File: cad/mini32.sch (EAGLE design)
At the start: 55 parts, among them CN1 MICROSDPLAIN, J1 HEADER-5X1, Q1 MOSFETSOT-23, SW2 SWITCHKMR211, SW3 SWITCHKMR211, U1 STM32F411/48, U2 LSM303D, U3 ADP5062, U4 MCP1824, U5 MAX17048, X1 12MHz, X2 32k768

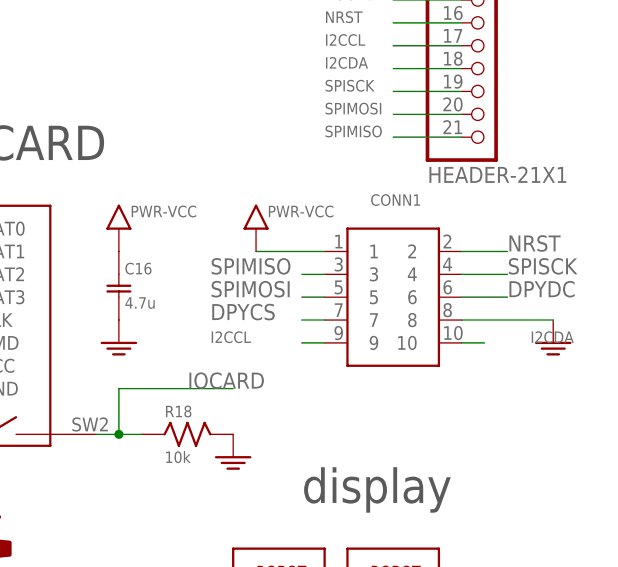
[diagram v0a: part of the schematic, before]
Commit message: 8pin dpy
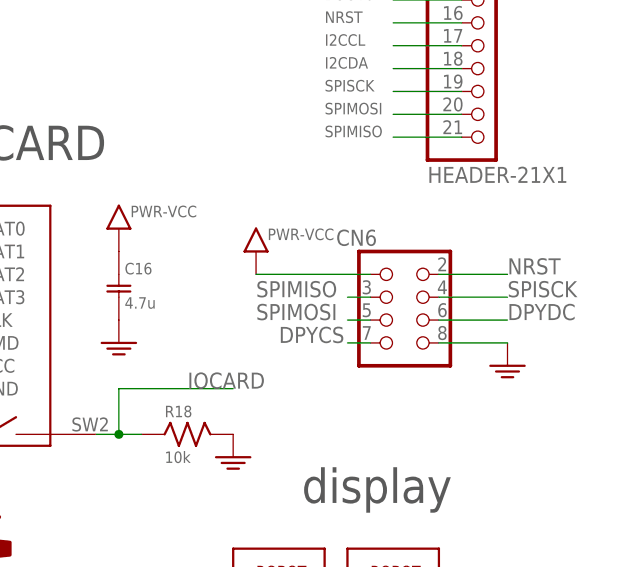
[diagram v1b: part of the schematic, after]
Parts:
- removed CONN1: HEADER-5X2-PTH, jaw:HEADER-5X2-PTH
- added CN6: (no value), jaw:HEADER-2X4
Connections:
- net DPYCS: now also CN6.P$7; no longer CONN1.7
- net DPYDC: now also CN6.P$6; no longer CONN1.6
- net GND: now also CN6.P$8; no longer CONN1.8
- net I2CCL: no longer CONN1.9
- net I2CDA: no longer CONN1.10
- net NRST: now also CN6.P$2; no longer CONN1.2
- net SPIMISO: now also CN6.P$3; no longer CONN1.3
- net SPIMOSI: now also CN6.P$5; no longer CONN1.5
- net SPISCK: now also CN6.P$4; no longer CONN1.4
- net VCC: now also CN6.P$1; no longer CONN1.1
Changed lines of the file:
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@@
 <setting verticaltext="up"/>
 </settings>
-<grid distance="0.1" unitdist="inch" unit="inch" style="lines" multiple="1" display="yes" altdistance="0.01" altunitdist="inch" altunit="inch"/>
+<grid distance="0.1" unitdist="inch" unit="inch" style="lines" multiple="1" display="no" altdistance="0.01" altunitdist="inch" altunit="inch"/>
 <layers>
 <layer number="1" name="Top" color="4" fill="1" visible="no" active="no"/>
@@
 <part name="GND19" library="jaw" deviceset="PWR-GND" device=""/>
 <part name="GND20" library="jaw" deviceset="PWR-GND" device=""/>
-<part name="GND24" library="jaw" deviceset="PWR-GND" device=""/>
-<part name="VCC20" library="jaw" deviceset="PWR-VCC" device=""/>
 <part name="J1" library="jaw" deviceset="HEADER-5X1" device=""/>
 <part name="U3" library="jaw" deviceset="ADP5062" device=""/>
@@
 <part name="U2" library="jaw" deviceset="LSM303D" device=""/>
 <part name="U5" library="jaw" deviceset="MAX17048" device=""/>
-<part name="CONN1" library="jaw" deviceset="HEADER-5X2" device="-PTH"/>
 <part name="LOGO1" library="Sparkfun-Aesthetics" deviceset="OSHW-LOGO" device="M"/>
 <part name="U$1" library="jaw" deviceset="ROBOTMAN-LOGO" device=""/>
 <part name="R2" library="jaw" deviceset="R" device="0603" value="100"/>
+<part name="CN6" library="jaw" deviceset="HEADER-2X4" device=""/>
+<part name="GND24" library="jaw" deviceset="PWR-GND" device=""/>
+<part name="VCC20" library="jaw" deviceset="PWR-VCC" device=""/>
 </parts>
 <sheets>
@@
 <instance part="GND19" gate="G$1" x="30.48" y="167.64"/>
 <instance part="GND20" gate="G$1" x="144.78" y="147.32"/>
-<instance part="GND24" gate="G$1" x="269.24" y="68.58"/>
-<instance part="VCC20" gate="G$1" x="236.22" y="81.28"/>
 <instance part="J1" gate="G$1" x="259.08" y="172.72"/>
 <instance part="U3" gate="G$1" x="35.56" y="50.8"/>
@@
 <instance part="U2" gate="G$1" x="99.06" y="106.68"/>
 <instance part="U5" gate="G$1" x="127" y="25.4"/>
-<instance part="CONN1" gate="G$1" x="251.46" y="68.58"/>
 <instance part="LOGO1" gate="G$1" x="203.2" y="45.72"/>
 <instance part="U$1" gate="G$1" x="238.76" y="40.64"/>
 <instance part="R2" gate="G$1" x="17.78" y="121.92"/>
+<instance part="CN6" gate="A" x="251.46" y="71.12"/>
+<instance part="GND24" gate="G$1" x="264.16" y="66.04"/>
+<instance part="VCC20" gate="G$1" x="236.22" y="78.74"/>
 </instances>
 <busses>
@@
 </segment>
 <segment>
-<pinref part="GND24" gate="G$1" pin="GND"/>
-<wire x1="269.24" y1="71.12" x2="259.08" y2="71.12" width="0.1524" layer="91"/>
-<pinref part="CONN1" gate="G$1" pin="8"/>
-</segment>
-<segment>
 <pinref part="JP1" gate="G$1" pin="12"/>
 <wire x1="259.08" y1="114.3" x2="251.46" y2="114.3" width="0.1524" layer="91"/>
@@
 <wire x1="142.24" y1="22.86" x2="147.32" y2="22.86" width="0.1524" layer="91"/>
 <label x="147.32" y="22.86" size="1.27" layer="95"/>
+</segment>
+<segment>
+<pinref part="CN6" gate="A" pin="P$8"/>
+<pinref part="GND24" gate="G$1" pin="GND"/>
+<wire x1="264.16" y1="68.58" x2="256.54" y2="68.58" width="0.1524" layer="91"/>
 </segment>
 </net>
@@
 </segment>
 <segment>
-<pinref part="VCC20" gate="G$1" pin="VCC"/>
-<wire x1="236.22" y1="78.74" x2="243.84" y2="78.74" width="0.1524" layer="91"/>
-<pinref part="CONN1" gate="G$1" pin="1"/>
-</segment>
-<segment>
 <pinref part="JP1" gate="G$1" pin="11"/>
 <wire x1="259.08" y1="116.84" x2="251.46" y2="116.84" width="0.1524" layer="91"/>
@@
 <wire x1="81.28" y1="116.84" x2="76.2" y2="116.84" width="0.1524" layer="91"/>
 <label x="73.66" y="116.84" size="1.27" layer="95"/>
+</segment>
+<segment>
+<pinref part="CN6" gate="A" pin="P$1"/>
+<pinref part="VCC20" gate="G$1" pin="VCC"/>
+<wire x1="236.22" y1="76.2" x2="248.92" y2="76.2" width="0.1524" layer="91"/>
 </segment>
 </net>
@@
 </segment>
 <segment>
-<label x="264.16" y="78.74" size="1.778" layer="95"/>
-<pinref part="CONN1" gate="G$1" pin="2"/>
-<wire x1="259.08" y1="78.74" x2="264.16" y2="78.74" width="0.1524" layer="91"/>
-</segment>
-<segment>
 <pinref part="J1" gate="G$1" pin="4"/>
 <wire x1="256.54" y1="170.18" x2="251.46" y2="170.18" width="0.1524" layer="91"/>
@@
 <wire x1="259.08" y1="104.14" x2="251.46" y2="104.14" width="0.1524" layer="91"/>
 <label x="243.84" y="104.14" size="1.27" layer="95"/>
+</segment>
+<segment>
+<pinref part="CN6" gate="A" pin="P$2"/>
+<wire x1="256.54" y1="76.2" x2="264.16" y2="76.2" width="0.1524" layer="91"/>
+<label x="264.16" y="76.2" size="1.778" layer="95"/>
 </segment>
 </net>
@@
 </segment>
 <segment>
-<label x="264.16" y="76.2" size="1.778" layer="95"/>
-<pinref part="CONN1" gate="G$1" pin="4"/>
-<wire x1="259.08" y1="76.2" x2="264.16" y2="76.2" width="0.1524" layer="91"/>
-</segment>
-<segment>
 <pinref part="JP1" gate="G$1" pin="19"/>
 <wire x1="259.08" y1="96.52" x2="251.46" y2="96.52" width="0.1524" layer="91"/>
 <label x="243.84" y="96.52" size="1.27" layer="95"/>
 </segment>
+<segment>
+<pinref part="CN6" gate="A" pin="P$4"/>
+<wire x1="256.54" y1="73.66" x2="264.16" y2="73.66" width="0.1524" layer="91"/>
+<label x="264.16" y="73.66" size="1.778" layer="95"/>
+</segment>
 </net>
 <net name="SPIMISO" class="0">
@@
 </segment>
 <segment>
-<pinref part="CONN1" gate="G$1" pin="3"/>
-<wire x1="243.84" y1="76.2" x2="241.3" y2="76.2" width="0.1524" layer="91"/>
-<label x="231.14" y="76.2" size="1.778" layer="95"/>
+<pinref part="CN6" gate="A" pin="P$3"/>
+<wire x1="248.92" y1="73.66" x2="246.38" y2="73.66" width="0.1524" layer="91"/>
+<label x="236.22" y="73.66" size="1.778" layer="95"/>
 </segment>
 </net>
@@
 </segment>
 <segment>
-<pinref part="CONN1" gate="G$1" pin="5"/>
-<wire x1="243.84" y1="73.66" x2="241.3" y2="73.66" width="0.1524" layer="91"/>
-<label x="231.14" y="73.66" size="1.778" layer="95"/>
+<pinref part="CN6" gate="A" pin="P$5"/>
+<wire x1="248.92" y1="71.12" x2="246.38" y2="71.12" width="0.1524" layer="91"/>
+<label x="236.22" y="71.12" size="1.778" layer="95"/>
 </segment>
 </net>
@@
 <label x="243.84" y="101.6" size="1.27" layer="95"/>
 </segment>
-<segment>
-<pinref part="CONN1" gate="G$1" pin="9"/>
-<wire x1="243.84" y1="68.58" x2="241.3" y2="68.58" width="0.1524" layer="91"/>
-<label x="231.14" y="68.58" size="1.27" layer="95"/>
-</segment>
 </net>
 <net name="I2CDA" class="0">
@@
 <label x="243.84" y="99.06" size="1.27" layer="95"/>
 </segment>
-<segment>
-<pinref part="CONN1" gate="G$1" pin="10"/>
-<wire x1="259.08" y1="68.58" x2="261.62" y2="68.58" width="0.1524" layer="91"/>
-<label x="266.7" y="68.58" size="1.27" layer="95"/>
-</segment>
 </net>
 <net name="DPYDC" class="0">
-<segment>
-<label x="264.16" y="73.66" size="1.778" layer="95"/>
-<pinref part="CONN1" gate="G$1" pin="6"/>
-<wire x1="259.08" y1="73.66" x2="264.16" y2="73.66" width="0.1524" layer="91"/>
-</segment>
 <segment>
 <pinref part="U1" gate="G$1" pin="PB10"/>
@@
 <label x="198.12" y="114.3" size="1.27" layer="95"/>
 </segment>
+<segment>
+<pinref part="CN6" gate="A" pin="P$6"/>
+<wire x1="256.54" y1="71.12" x2="264.16" y2="71.12" width="0.1524" layer="91"/>
+<label x="264.16" y="71.12" size="1.778" layer="95"/>
+</segment>
 </net>
 <net name="DPYCS" class="0">
@@
 </segment>
 <segment>
-<pinref part="CONN1" gate="G$1" pin="7"/>
-<wire x1="243.84" y1="71.12" x2="241.3" y2="71.12" width="0.1524" layer="91"/>
-<label x="231.14" y="71.12" size="1.778" layer="95"/>
-</segment>
-</net>
+<pinref part="CN6" gate="A" pin="P$7"/>
+<wire x1="248.92" y1="68.58" x2="246.38" y2="68.58" width="0.1524" layer="91"/>
+<label x="238.76" y="68.58" size="1.778" layer="95"/>
+</segment>
+</net>
